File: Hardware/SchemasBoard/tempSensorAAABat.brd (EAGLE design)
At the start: 20.2 x 15.4 mm, 10 parts, among them IC1 DS1820

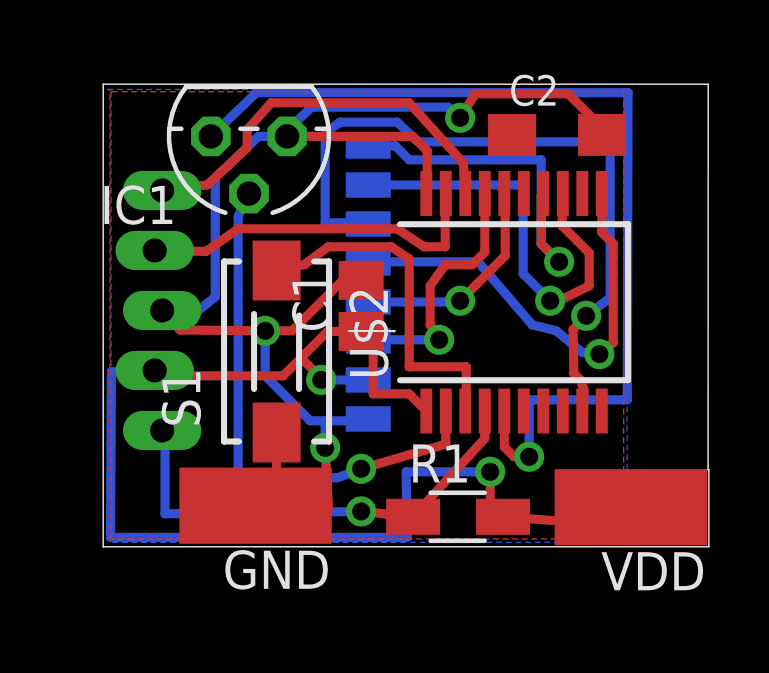
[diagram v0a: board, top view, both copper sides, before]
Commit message: change in the layout
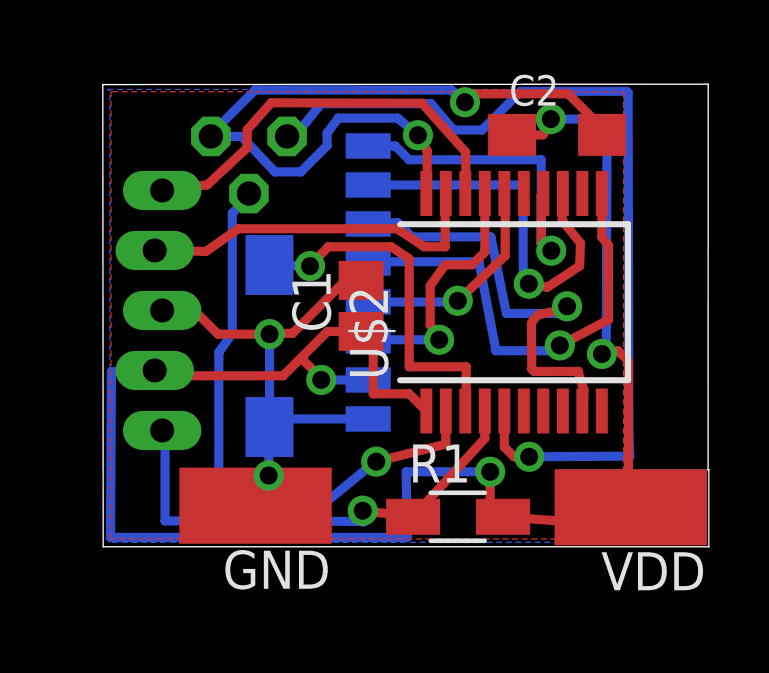
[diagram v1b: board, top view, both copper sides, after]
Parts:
- moved S1 0.30 mm to (5.54, 6.70), flipped to the bottom
- flipped IC1 to the bottom
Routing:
- net VDD: track 42.9 -> 60.2 mm, vias 2 -> 4
- net N$23: track 23.8 -> 14.9 mm
- net GND: track 49.0 -> 42.6 mm, vias 3 -> 4
- net N$1: track 18.4 -> 20.0 mm
- net N$3: track 32.1 -> 30.5 mm
- net N$12: track 14.3 -> 13.1 mm
- net N$21: track 12.2 -> 11.3 mm
- net N$25: track 15.5 -> 16.2 mm
- net N$2: track 11.7 -> 12.0 mm, vias 0 -> 1
